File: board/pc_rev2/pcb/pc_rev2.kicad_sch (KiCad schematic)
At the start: 18 parts, among them J1 Conn_02x13_Odd_Even, J11 Conn_01x03, J2 Conn_02x08_Row_Letter_Last, J3 Conn_02x06_Row_Letter_Last, J4 Conn_02x10_Row_Letter_Last, J5 Conn_Grove_Host, J6 Conn_Grove-Analog_Host, J7 Conn_Grove-Analog_Host, J8 Conn_01x05, U2 AE-FT234X

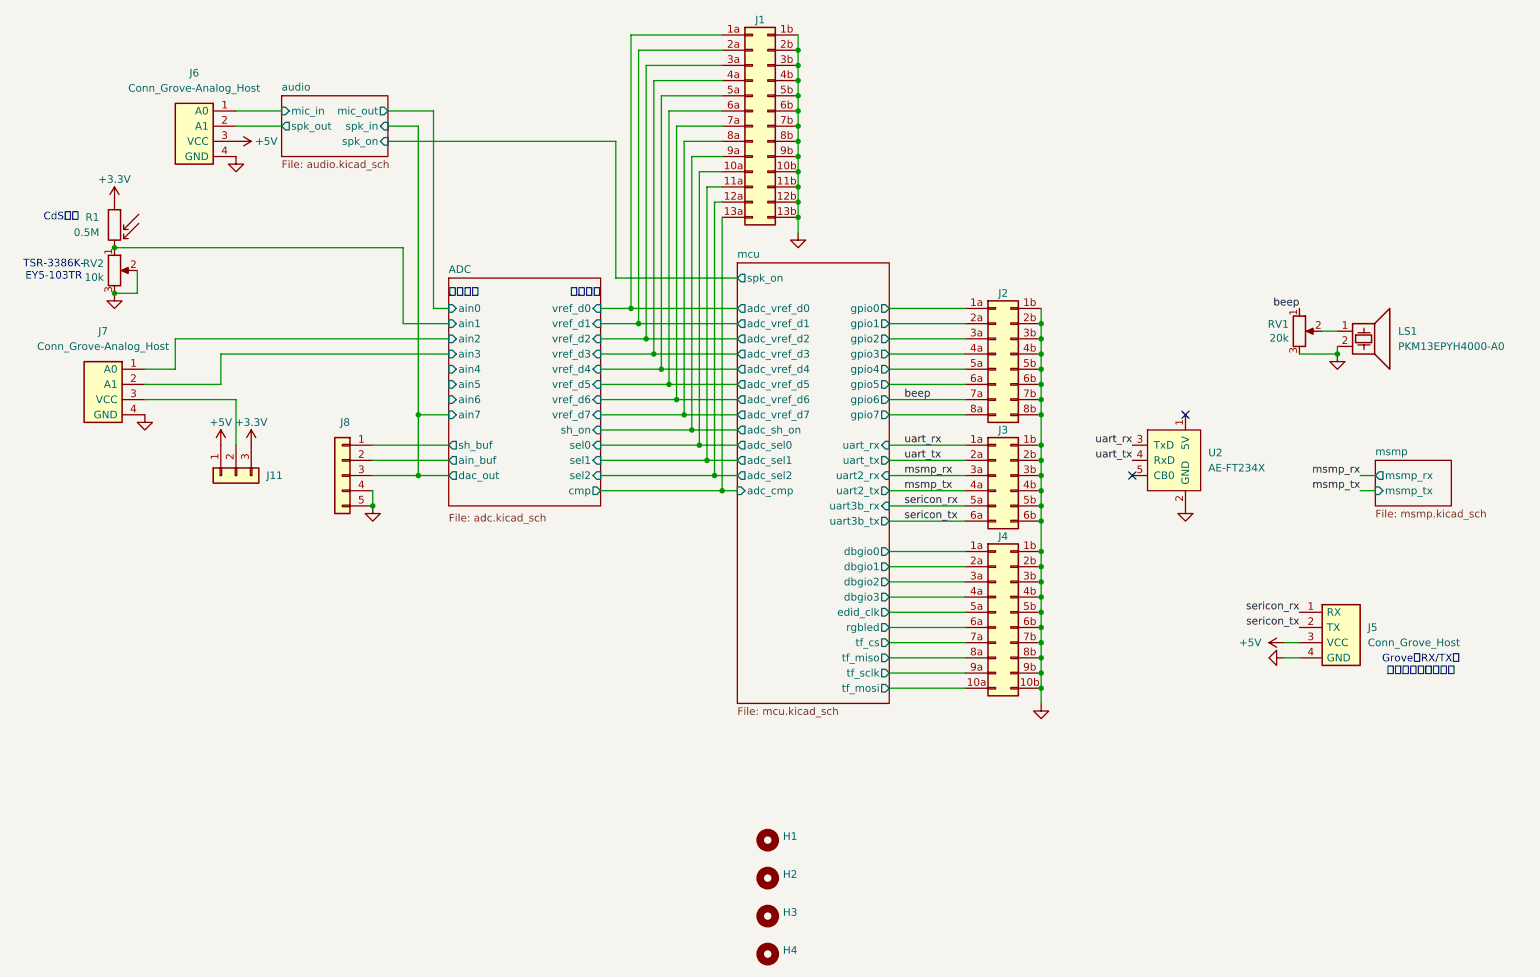
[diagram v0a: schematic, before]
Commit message: 諸々改良＆基板デザイン（WIP）
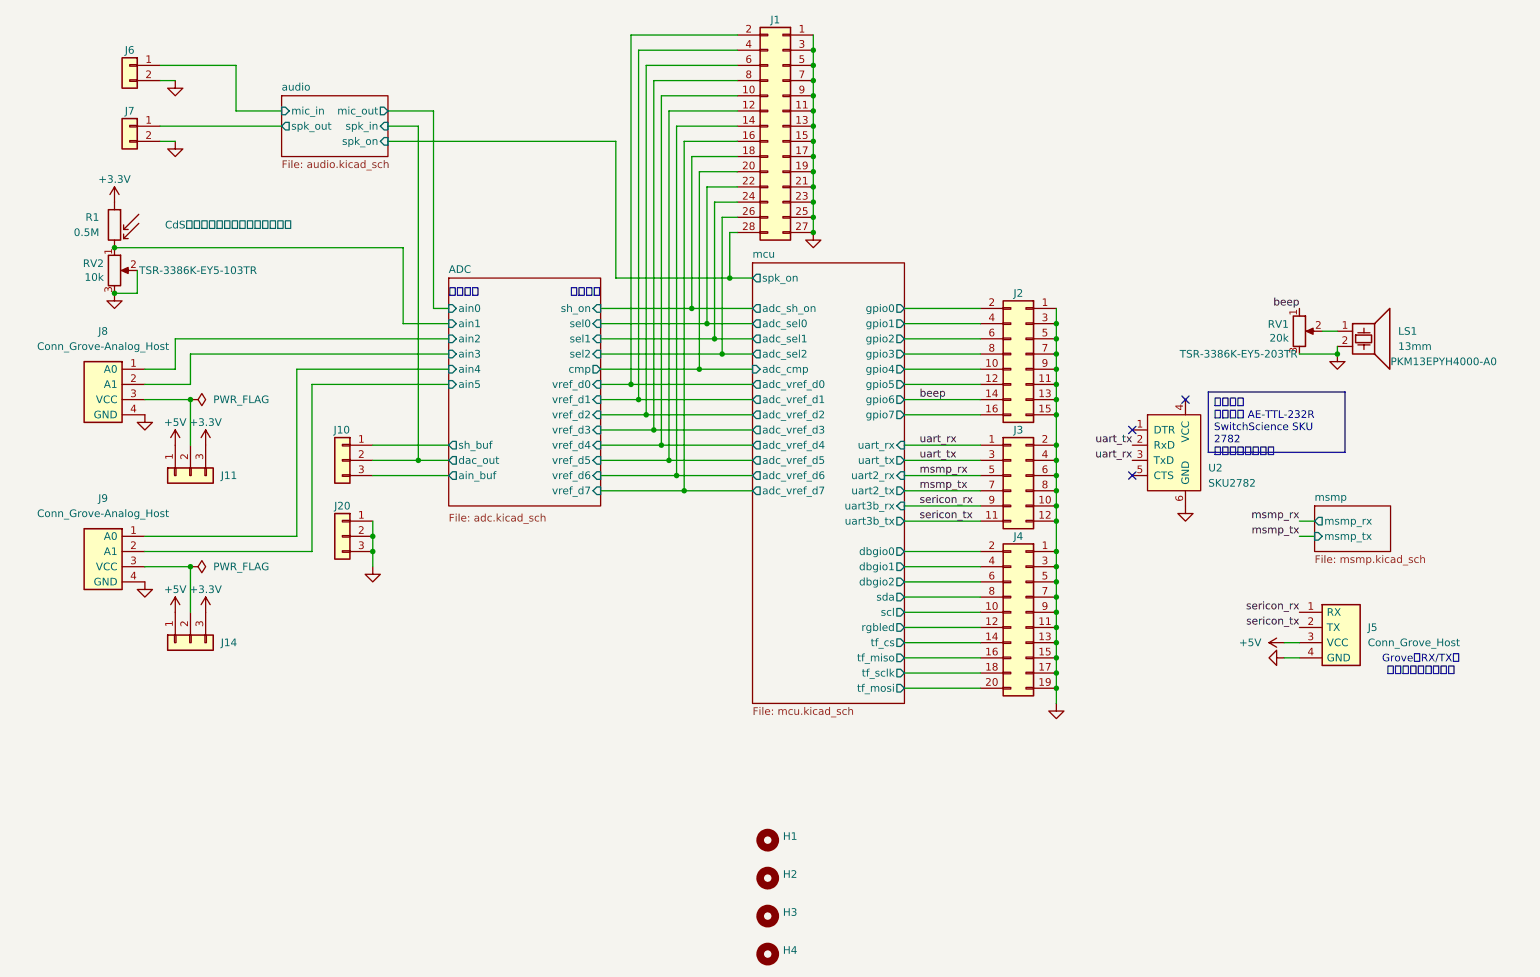
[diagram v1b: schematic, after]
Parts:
- removed J6: Conn_Grove-Analog_Host, uchan:Grove_1x04_P2mm_THT_Horizontal, symbol uchan:Conn_Grove-Analog_Host
- removed U2: AE-FT234X, uchan:AE-FT234X, symbol uchan:AE-FT234X
- added J14, J20: Conn_01x03, Connector_PinHeader_2.54mm:PinHeader_1x03_P2.54mm_Vertical, symbol Connector_Generic:Conn_01x03
- added J6, J7: Conn_01x03, Connector_JST:JST_XH_S2B-XH-A_1x02_P2.50mm_Horizontal, symbol Connector_Generic:Conn_01x02
- added J9: Conn_Grove-Analog_Host, uchan:Grove_1x04_P2mm_THT_Horizontal, symbol uchan:Conn_Grove-Analog_Host
- added U2: SKU2782, uchan:SKU2782, symbol uchan:SKU2782
- J1: footprint (none) -> Connector_PinHeader_2.54mm:PinHeader_2x14_P2.54mm_Vertical; symbol Connector_Generic:Conn_02x13_Row_Letter_Last -> Connector_Generic:Conn_02x14_Odd_Even
- J10: renamed from J8; footprint Connector_PinHeader_2.54mm:PinHeader_1x05_P2.54mm_Vertical -> Connector_PinHeader_2.54mm:PinHeader_1x03_P2.54mm_Vertical; symbol Connector_Generic:Conn_01x05 -> Connector_Generic:Conn_01x03
- J2: footprint (none) -> Connector_PinHeader_2.54mm:PinHeader_2x08_P2.54mm_Vertical; symbol Connector_Generic:Conn_02x08_Row_Letter_Last -> Connector_Generic:Conn_02x08_Odd_Even
- J3: footprint (none) -> Connector_PinHeader_2.54mm:PinHeader_2x06_P2.54mm_Vertical; symbol Connector_Generic:Conn_02x06_Row_Letter_Last -> Connector_Generic:Conn_02x06_Odd_Even
- J4: footprint (none) -> Connector_PinHeader_2.54mm:PinHeader_2x10_P2.54mm_Vertical; symbol Connector_Generic:Conn_02x10_Row_Letter_Last -> Connector_Generic:Conn_02x10_Odd_Even
- LS1: value PKM13EPYH4000-A0 -> 13mm; Manufacturer (none) -> Murata; Manufacturer PN (none) -> PKM13EPYH4000-A0
- R1: Manufacturer (none) -> Senba; Manufacturer PN (none) -> GL5516; Purpose (none) -> CdSセル。周辺の明るさを取得する
- RV1: footprint Potentiometer_SMD:Potentiometer_Bourns_TC33X_Vertical -> uchan:Potentiometer_Suntan_TSR-3386K_Vertical; Manufacturer (none) -> Suntan; Manufacturer PN (none) -> TSR-3386K-EY5-203TR
- RV2: Manufacturer (none) -> SUNTAN; Manufacturer PN (none) -> TSR-3386K-EY5-103TR
- renumbered J7 to J8
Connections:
- net ADC/ain7 is gone; now on net ADC/ain_buf: J10.3 (Pin_3)
- net +3.3V: now also J14.3 (Pin_3)
- net +5V: now also J14.1 (Pin_1)
- net ADC/ain4: now also J9.1 (A0)
- net ADC/ain5: now also J9.2 (A1)
- net ADC/ain_buf: no longer J10.2 (Pin_2)
- net ADC/cmp: now also J1.20 (Pin_20); no longer J1.13a (Pin_13a)
- net ADC/sel0: now also J1.22 (Pin_22); no longer J1.10a (Pin_10a)
- net ADC/sel1: now also J1.24 (Pin_24); no longer J1.11a (Pin_11a)
- net ADC/sel2: now also J1.26 (Pin_26); no longer J1.12a (Pin_12a)
- net ADC/sh_on: now also J1.18 (Pin_18); no longer J1.9a (Pin_9a)
- net ADC/vref_d0: now also J1.2 (Pin_2); no longer J1.1a (Pin_1a)
- net ADC/vref_d1: now also J1.4 (Pin_4); no longer J1.2a (Pin_2a)
- net ADC/vref_d2: now also J1.6 (Pin_6); no longer J1.3a (Pin_3a)
- net ADC/vref_d3: now also J1.8 (Pin_8); no longer J1.4a (Pin_4a)
- net ADC/vref_d4: now also J1.10 (Pin_10); no longer J1.5a (Pin_5a)
- net ADC/vref_d5: now also J1.12 (Pin_12); no longer J1.6a (Pin_6a)
- net ADC/vref_d6: now also J1.14 (Pin_14); no longer J1.7a (Pin_7a)
- net ADC/vref_d7: now also J1.16 (Pin_16); no longer J1.8a (Pin_8a)
- net GND: now also J1.1 (Pin_1), J1.11 (Pin_11), J1.13 (Pin_13), J1.15 (Pin_15), J1.17 (Pin_17), J1.19 (Pin_19), J1.21 (Pin_21), J1.23 (Pin_23), J1.25 (Pin_25), J1.27 (Pin_27), J1.3 (Pin_3), J1.5 (Pin_5), J1.7 (Pin_7), J1.9 (Pin_9), J2.1 (Pin_1), J2.11 (Pin_11), J2.13 (Pin_13), J2.15 (Pin_15), J2.3 (Pin_3), J2.5 (Pin_5), J2.7 (Pin_7), J2.9 (Pin_9), J3.10 (Pin_10), J3.12 (Pin_12), J3.2 (Pin_2), J3.4 (Pin_4), J3.6 (Pin_6), J3.8 (Pin_8), J4.1 (Pin_1), J4.11 (Pin_11), J4.13 (Pin_13), J4.15 (Pin_15), J4.17 (Pin_17), J4.19 (Pin_19), J4.3 (Pin_3), J4.5 (Pin_5), J4.7 (Pin_7), J4.9 (Pin_9), J20.1 (Pin_1), J20.2 (Pin_2), J20.3 (Pin_3), J6.2 (Pin_2), J7.2 (Pin_2), J9.4 (GND), U2.6 (GND); no longer J1.10b (Pin_10b), J1.11b (Pin_11b), J1.12b (Pin_12b), J1.13b (Pin_13b), J1.1b (Pin_1b), J1.2b (Pin_2b), J1.3b (Pin_3b), J1.4b (Pin_4b), J1.5b (Pin_5b), J1.6b (Pin_6b), J1.7b (Pin_7b), J1.8b (Pin_8b), J1.9b (Pin_9b), J10.4 (Pin_4), J10.5 (Pin_5), J2.1b (Pin_1b), J2.2b (Pin_2b), J2.3b (Pin_3b), J2.4b (Pin_4b), J2.5b (Pin_5b), J2.6b (Pin_6b), J2.7b (Pin_7b), J2.8b (Pin_8b), J3.1b (Pin_1b), J3.2b (Pin_2b), J3.3b (Pin_3b), J3.4b (Pin_4b), J3.5b (Pin_5b), J3.6b (Pin_6b), J4.10b (Pin_10b), J4.1b (Pin_1b), J4.2b (Pin_2b), J4.3b (Pin_3b), J4.4b (Pin_4b), J4.5b (Pin_5b), J4.6b (Pin_6b), J4.7b (Pin_7b), J4.8b (Pin_8b), J4.9b (Pin_9b)
- net audio/mic_in: now also J6.1 (Pin_1)
- net audio/spk_on: now also J1.28 (Pin_28)
- net audio/spk_out: now also J7.1 (Pin_1)
- net beep: now also J2.14 (Pin_14); no longer J2.7a (Pin_7a)
- net mcu/dbgio0: now also J4.2 (Pin_2); no longer J4.1a (Pin_1a)
- net mcu/dbgio1: now also J4.4 (Pin_4); no longer J4.2a (Pin_2a)
- net mcu/dbgio2: now also J4.6 (Pin_6); no longer J4.3a (Pin_3a)
- net mcu/gpio0: now also J2.2 (Pin_2); no longer J2.1a (Pin_1a)
- net mcu/gpio1: now also J2.4 (Pin_4); no longer J2.2a (Pin_2a)
- net mcu/gpio2: now also J2.6 (Pin_6); no longer J2.3a (Pin_3a)
- net mcu/gpio3: now also J2.8 (Pin_8); no longer J2.4a (Pin_4a)
- net mcu/gpio4: now also J2.10 (Pin_10); no longer J2.5a (Pin_5a)
- net mcu/gpio5: now also J2.12 (Pin_12); no longer J2.6a (Pin_6a)
- net mcu/gpio7: now also J2.16 (Pin_16); no longer J2.8a (Pin_8a)
- net mcu/rgbled: now also J4.12 (Pin_12); no longer J4.6a (Pin_6a)
- net mcu/tf_cs: now also J4.14 (Pin_14); no longer J4.7a (Pin_7a)
- net mcu/tf_miso: now also J4.16 (Pin_16); no longer J4.8a (Pin_8a)
- net mcu/tf_mosi: now also J4.20 (Pin_20); no longer J4.10a (Pin_10a)
- net mcu/tf_sclk: now also J4.18 (Pin_18); no longer J4.9a (Pin_9a)
- net msmp_rx: now also J3.5 (Pin_5); no longer J3.3a (Pin_3a)
- net msmp_tx: now also J3.7 (Pin_7); no longer J3.4a (Pin_4a)
- net sericon_rx: now also J3.9 (Pin_9); no longer J3.5a (Pin_5a)
- net sericon_tx: now also J3.11 (Pin_11); no longer J3.6a (Pin_6a)
- net uart_rx: now also J3.1 (Pin_1), U2.3 (TxD); no longer J3.1a (Pin_1a)
- net uart_tx: now also J3.3 (Pin_3), U2.2 (RxD); no longer J3.2a (Pin_2a)
- removed net mcu/dbgio3: J4.4a (Pin_4a)
- removed net mcu/edid_clk: J4.5a (Pin_5a)
- new net: J14.2 (Pin_2), J9.3 (VCC)
- new net ADC/dac_out: J10.2 (Pin_2)
- new net mcu/scl: J4.10 (Pin_10)
- new net mcu/sda: J4.8 (Pin_8)
- no-connect marks 2 -> 3
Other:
- sheet ADC ports: added none; removed ain6, ain7
- sheet mcu ports: added scl, sda; removed dbgio3, edid_clk
- note removed: "CdSセル"
- note removed: "TSR-3386K- EY5-103TR"
- moved on the sheet: J11, J2, J3, J4
